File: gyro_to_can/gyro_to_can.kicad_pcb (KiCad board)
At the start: 2 copper layers, 52 x 55 mm, 22 parts, among them J101 PWR, J201 can, P1 Digital, P2 Analog, P3 CONN_01X01, P4 CONN_01X01, P5 CONN_01X01, P6 CONN_01X01, U101 MPU6050_module, U201 PESD5V0L2UU_esd_diode, U202 MCP2551-I-SN, U203 MCP2515-xST, Y201 Crystal

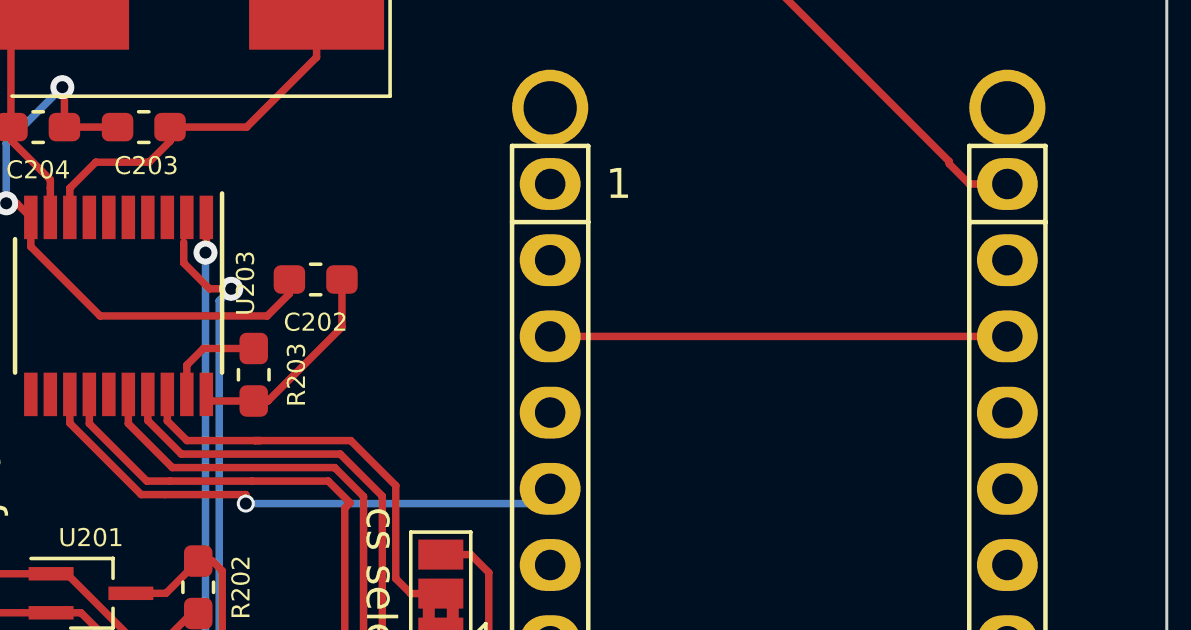
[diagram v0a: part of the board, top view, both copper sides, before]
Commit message: initial
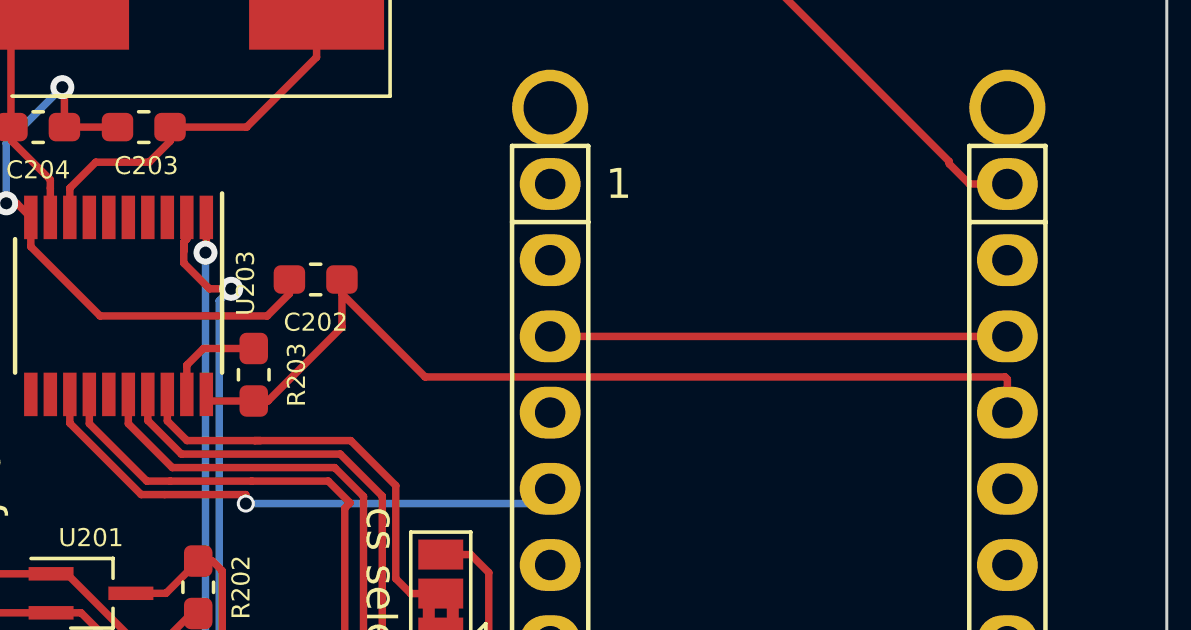
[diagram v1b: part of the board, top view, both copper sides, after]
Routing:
- net +5V: track 9.55 -> 34.5 mm
- net /Sheet60784F27/can_rx: track 21.7 -> 22.9 mm
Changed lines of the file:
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@@
     (thickness 1.6)
     (drawings 28)
-    (tracks 216)
+    (tracks 224)
     (zones 0)
     (modules 22)
@@
     (visible_elements FFFFFF7F)
     (pcbplotparams
-      (layerselection 0x00030_80000001)
+      (layerselection 0x010f0_ffffffff)
       (usegerberextensions false)
       (usegerberattributes false)
@@
       (outputformat 1)
       (mirror false)
-      (drillshape 1)
+      (drillshape 0)
       (scaleselection 1)
-      (outputdirectory ""))
+      (outputdirectory "../../gerb_out/"))
   )
   (net 0 "")
@@
   (segment (start 132.504999 76.015001) (end 130.039999 78.480001) (width 0.25) (layer F.Cu) (net 15))
   (segment (start 130.039999 78.480001) (end 129.564999 78.480001) (width 0.25) (layer F.Cu) (net 15))
+  (segment (start 132.504999 74.905001) (end 132.504999 74.430001) (width 0.25) (layer F.Cu) (net 15))
+  (segment (start 135.278388 77.67839) (end 132.504999 74.905001) (width 0.25) (layer F.Cu) (net 15))
+  (segment (start 154.61099 77.67839) (end 135.278388 77.67839) (width 0.25) (layer F.Cu) (net 15))
+  (segment (start 154.686 77.7534) (end 154.61099 77.67839) (width 0.25) (layer F.Cu) (net 15))
+  (segment (start 154.686 78.867) (end 154.686 77.7534) (width 0.25) (layer F.Cu) (net 15))
   (segment (start 127.38 100) (end 127.38 104.68) (width 0.25) (layer F.Cu) (net 18))
   (segment (start 127.38 104.68) (end 135.1 112.4) (width 0.25) (layer F.Cu) (net 18))
@@
   (segment (start 127.144999 91.670001) (end 127.114999 91.640001) (width 0.25) (layer F.Cu) (net 41))
   (via (at 127.114999 91.640001) (size 0.8) (drill 0.4) (layers F.Cu B.Cu) (net 41))
+  (segment (start 127.232318 73.186599) (end 127.232318 73.5) (width 0.25) (layer F.Cu) (net 41))
+  (segment (start 127.334999 73.083918) (end 127.232318 73.186599) (width 0.25) (layer F.Cu) (net 41))
+  (segment (start 127.334999 72.360001) (end 127.334999 73.083918) (width 0.25) (layer F.Cu) (net 41))
   (segment (start 123.264999 91.490001) (end 123.264999 93.045001) (width 0.25) (layer F.Cu) (net 42))
   (segment (start 123.264999 93.045001) (end 123.334999 93.115001) (width 0.25) (layer F.Cu) (net 42))
